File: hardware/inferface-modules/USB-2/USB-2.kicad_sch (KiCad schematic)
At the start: 9 parts, among them J1 USB_device, J2 USB_PT, J3 Base_Board_Interface

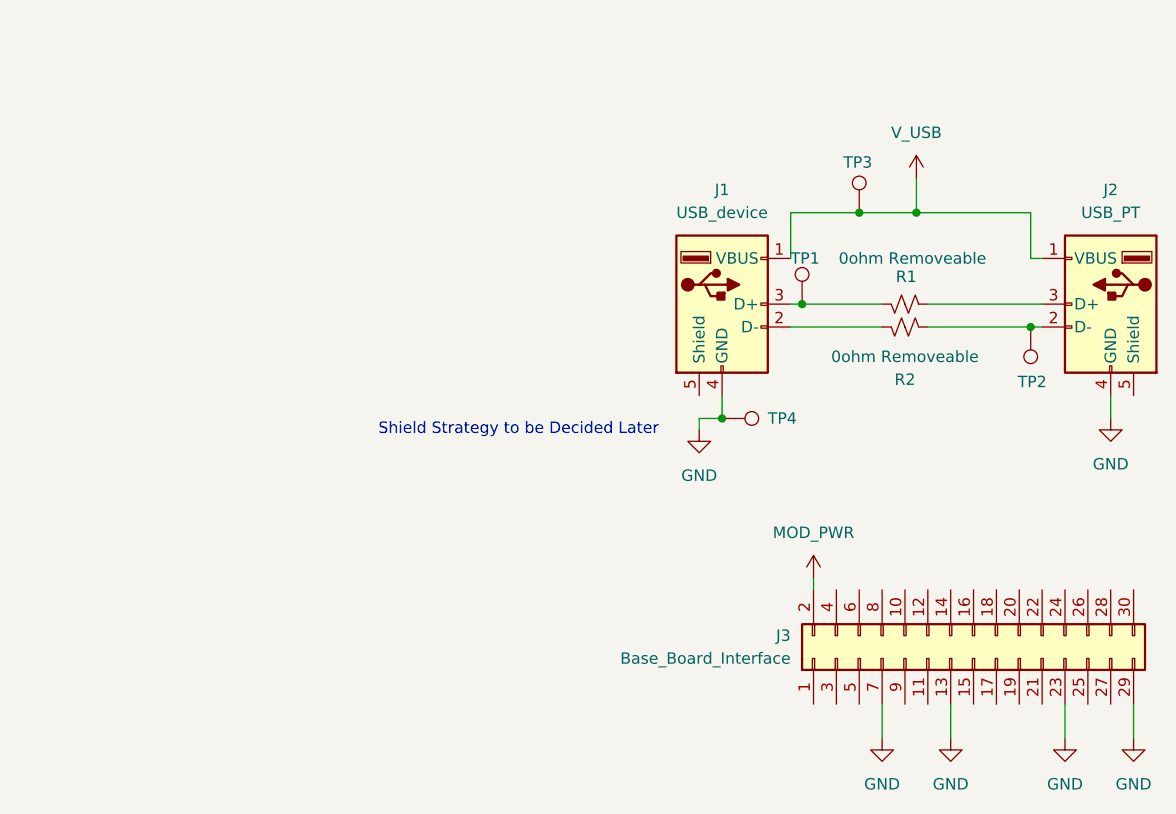
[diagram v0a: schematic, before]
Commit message: esd array implemented
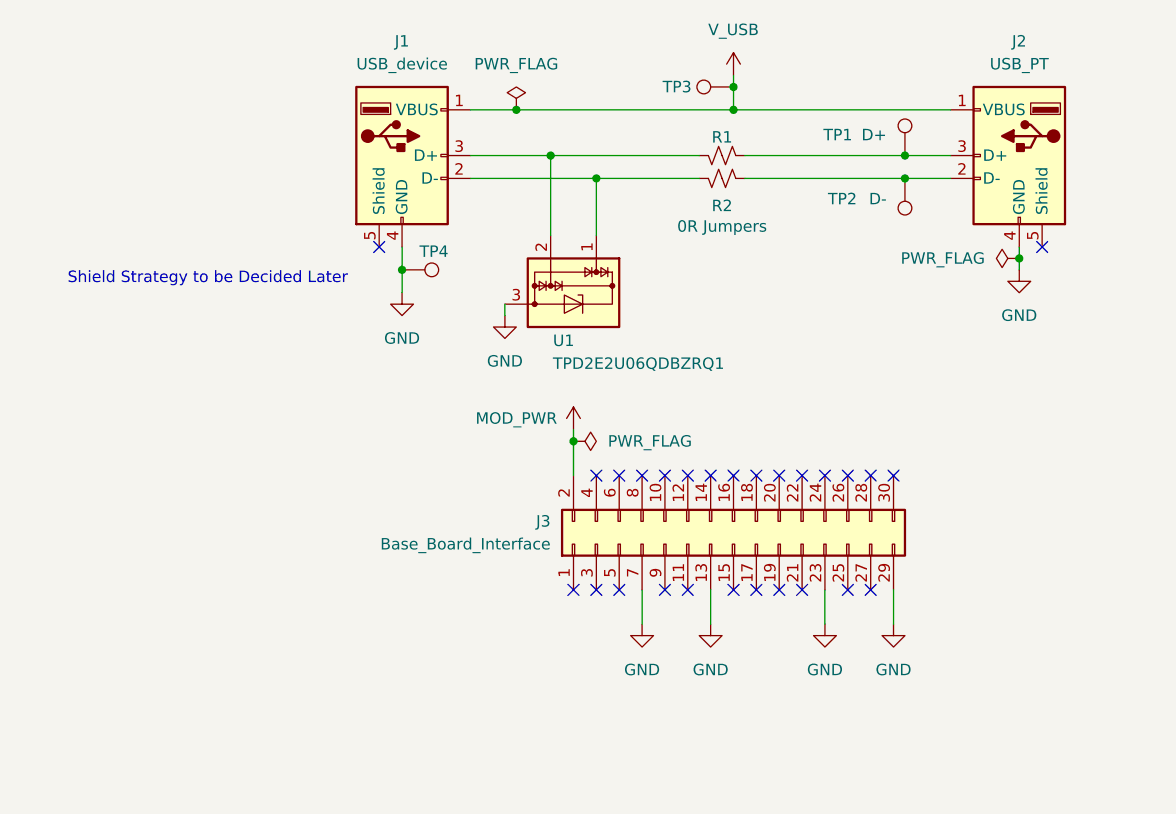
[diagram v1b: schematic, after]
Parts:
- added U1: TPD2E2U06QDBZRQ1, Package_TO_SOT_SMD:SOT-23, symbol Power_Protection:TPD2E2U06DCK
- R1: value 0ohm Removeable -> R_Small_US; footprint (none) -> Resistor_SMD:R_0805_2012Metric
- R2: value 0ohm Removeable -> 0R Jumpers; footprint (none) -> Resistor_SMD:R_0805_2012Metric
- TP1: value TestPoint -> D+; footprint (none) -> TestPoint:TestPoint_Pad_1.0x1.0mm
- TP2: value TestPoint -> D-; footprint (none) -> TestPoint:TestPoint_Pad_1.0x1.0mm
- TP3, TP4: footprint (none) -> TestPoint:TestPoint_Pad_1.0x1.0mm
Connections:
- net GND: now also U1.3
- net at J1.2 (D-), R2.1: now also U1.1
- net at R1.2, TP1.1: now also J2.3 (D+); no longer J1.3 (D+)
- net at R1.1: now also J1.3 (D+), U1.2; no longer J2.3 (D+)
- no-connect marks 0 -> 27
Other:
- moved on the sheet: J1, J2, J3, TP3
